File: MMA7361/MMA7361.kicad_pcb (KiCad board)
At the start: 2 copper layers, 23.4 x 22.9 mm, 13 parts, among them J1 Conn_01x05, J2 Conn_01x05, U1 RT9701, U2 MMA7260Q

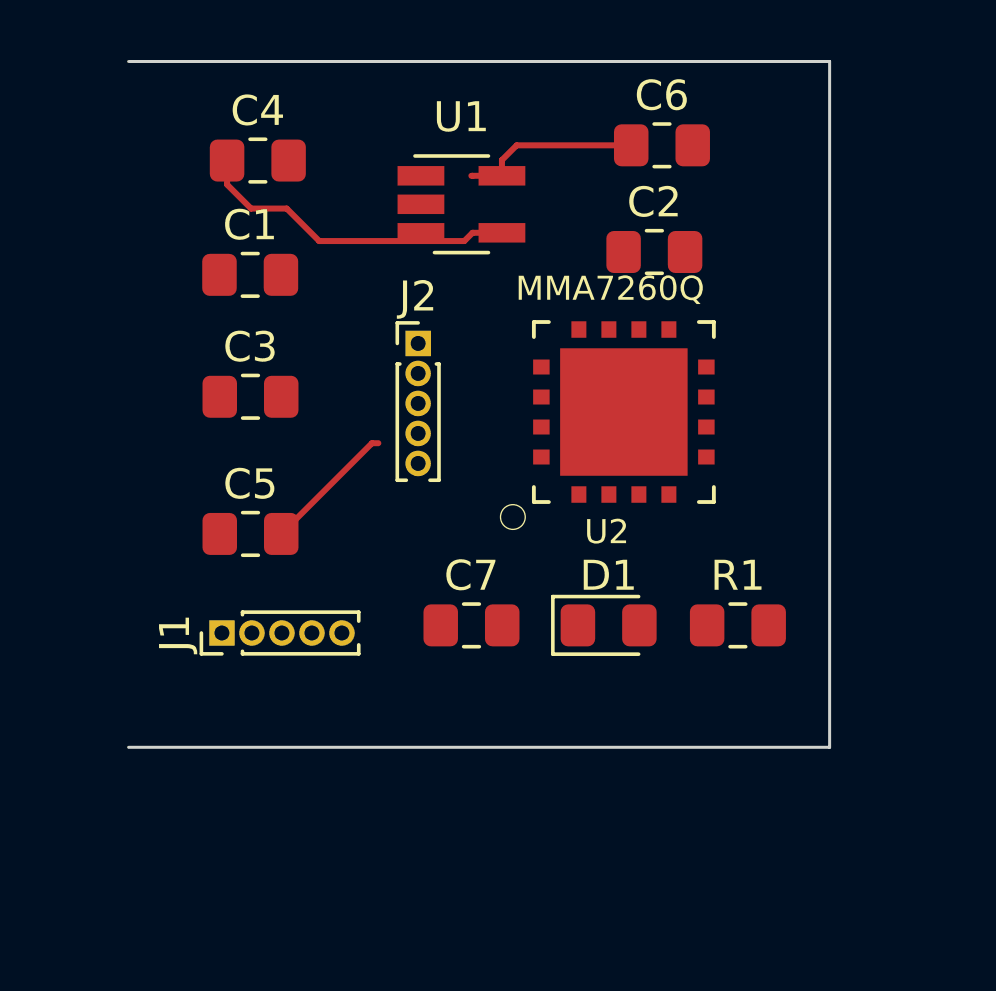
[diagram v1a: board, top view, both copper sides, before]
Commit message: More changes
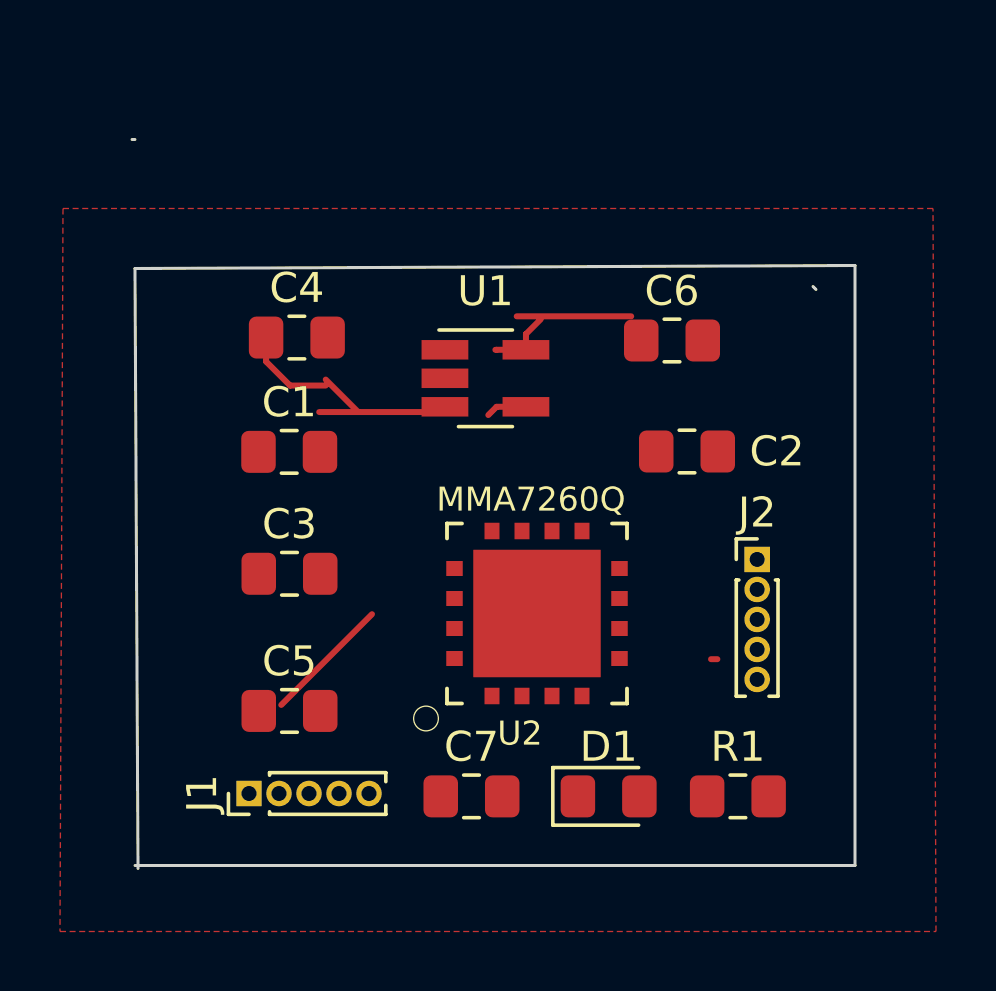
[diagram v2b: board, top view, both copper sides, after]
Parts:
- moved J2 13.4 mm to (150.2, 92.8)
- moved U2 7.31 mm to (142.9, 94.6)
- moved C2 6.74 mm to (147.9, 89.2)
- moved C6 6.51 mm to (147.4, 85.5)
- moved C4 6.04 mm to (134.9, 85.4)
- moved C5 6.04 mm to (134.7, 97.8)
- moved C1 6.04 mm to (134.6, 89.2)
- moved C3 6.04 mm to (134.7, 93.3)
- moved U1 5.85 mm to (141.2, 86.8)
- moved C7 5.70 mm to (140.7, 100.7)
- moved D1 5.70 mm to (145.3, 100.7)
- moved R1 5.70 mm to (149.6, 100.7)
- moved J1 5.43 mm to (133.3, 100.6)
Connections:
- C1 pad 2: /MMA 7361 Module/X -> Net-(C1-Pad2)
- C3 pad 2: /MMA 7361 Module/Y -> Net-(C3-Pad2)
- C5 pad 2: /MMA 7361 Module/Z -> Net-(C5-Pad2)
- C6 pad 1: /MMA 7361 Module/VCC -> VCC
- C7 pad 1: GND -> VCC
- C7 pad 2: /MMA 7361 Module/VCC -> GND
- J1 pad 2: /MMA 7361 Module/VCC -> VCC
- J1 pad 5: Net-(J1-Pad5) -> /MMA 7361 Module/SelfTest
- J2 pad 1: /MMA 7361 Module/X -> GND
- J2 pad 2: /MMA 7361 Module/Y -> GND
- J2 pad 3: /MMA 7361 Module/Z -> GND
- R1 pad 2: /MMA 7361 Module/VCC -> VCC
- U1 pad 1: /MMA 7361 Module/VCC -> VCC
- U1 pad 5: /MMA 7361 Module/VCC -> VCC
- U2 pad 1: /MMA 7361 Module/Og-Detect -> Net-(U2-Pad1)
- U2 pad 10: (no net) -> /MMA 7361 Module/g-Select
- U2 pad 11: (no net) -> Net-(U2-Pad11)
- U2 pad 12: /MMA 7361 Module/Sleep -> Net-(U2-Pad12)
- U2 pad 13: /MMA 7361 Module/Z -> /MMA 7361 Module/SelfTest
- U2 pad 14: /MMA 7361 Module/Y -> (no net)
- U2 pad 15: /MMA 7361 Module/X -> (no net)
- U2 pad 2: /MMA 7361 Module/g-Select -> Net-(C3-Pad2)
- U2 pad 3: /MMA 7361 Module/VCC -> Net-(C5-Pad2)
- U2 pad 4: GND -> Net-(C1-Pad2)
- U2 pad 5: (no net) -> GND
- U2 pad 6: (no net) -> VCC
- U2 pad 7: (no net) -> /MMA 7361 Module/Sleep
- U2 pad 8: (no net) -> Net-(U2-Pad8)
- U2 pad 9: (no net) -> /MMA 7361 Module/Og-Detect
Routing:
- net /MMA 7361 Module/VCC: track 6.06 -> 0.00 mm
- net VCC: track 0.00 -> 6.06 mm
- net Net-(C5-Pad2): track 0.00 -> 4.49 mm
- net /MMA 7361 Module/Z: track 4.49 -> 0.00 mm
- added copper zone on F.Cu, net GND
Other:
- board size 23.4 x 22.9 mm -> 24.1 x 24.3 mm
- net class Default: clearance 0.8 -> 0.25; trace_width 0.2 -> 0.25; via_drill 0.6 -> 0.5
- net class Test removed
- rule trace_clearance: 0.8 -> 0.25
- rule trace_min: 0.2 -> 0.25
- rule via_min_drill: 0.3 -> 0.5
- rule via_min_size: 0.4 -> 1
